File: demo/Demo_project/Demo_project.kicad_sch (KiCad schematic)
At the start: 58 parts, among them J1 USB_C_Receptacle_USB2.0, J2 Conn_01x04, J3 Screw_Terminal_01x03, J4 Screw_Terminal_01x08, J5 Screw_Terminal_01x02, K1 RT314A05, Q1 UMH3N, Q2 BC817, SW1 SW_SPST, U1 ESP32-WROOM-32D, U2 USBLC6-2P6, U3 CP2104, U4 Si7021-A20, U5 74AHCT245, U6 TLV1117LV-3.3

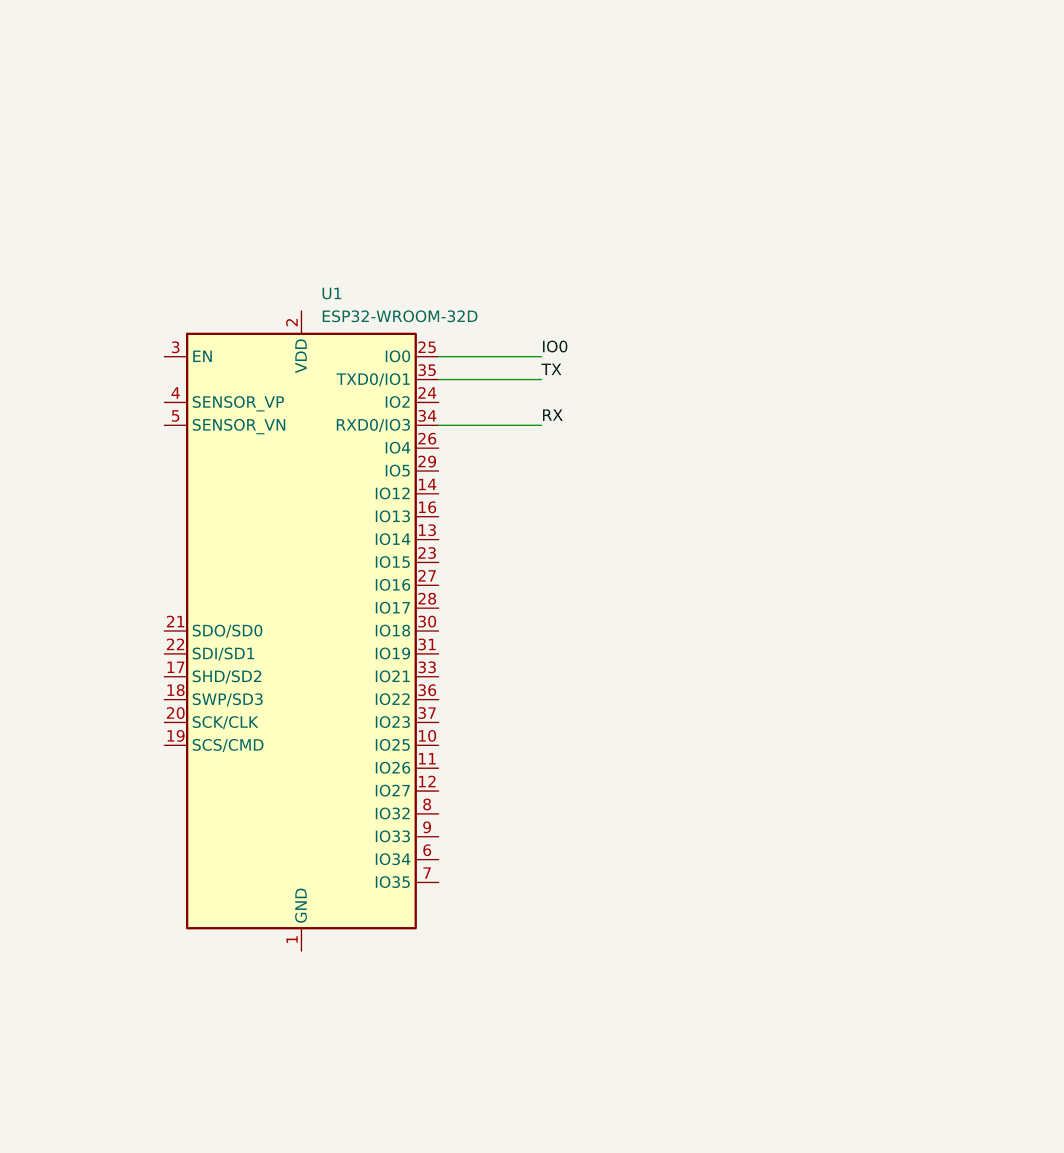
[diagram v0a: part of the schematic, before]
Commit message: v0.1 beta
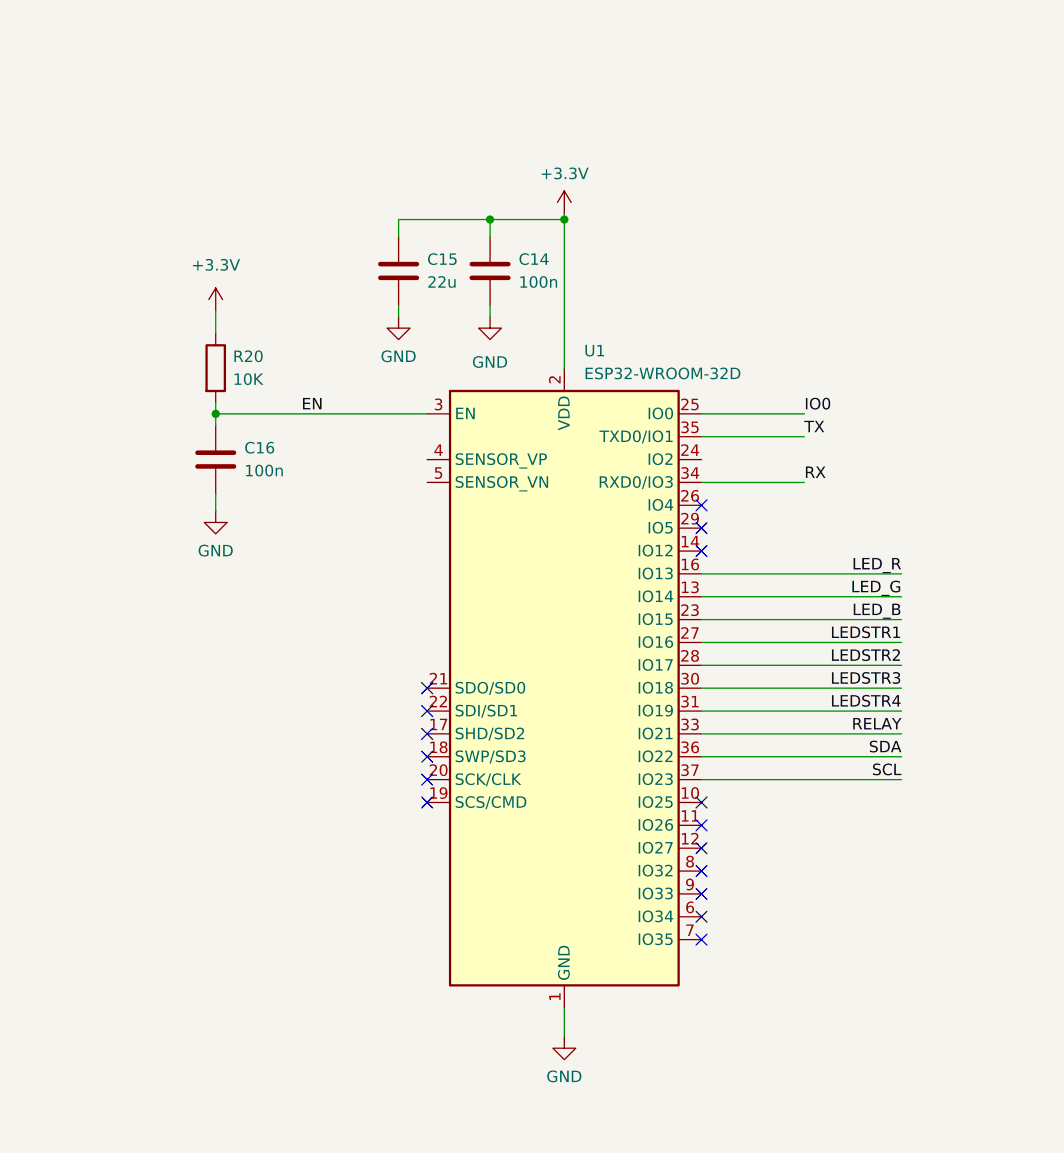
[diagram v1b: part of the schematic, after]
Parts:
- added C14, C16: 100n, symbol Device:C
- added C15: 22u, symbol Device:C
- added R20: 10K, symbol Device:R
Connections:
- net +3.3V: now also U1.2 (VDD), C14.1, C15.1, R20.1
- net EN: now also U1.3 (EN), C16.1, R20.2
- net GND: now also U1.1 (GND), U1.15 (GND), U1.38 (GND), U1.39 (GND), C14.2, C15.2, C16.2
- net LEDSTR1: now also U1.27 (IO16)
- net LEDSTR2: now also U1.28 (IO17)
- net LEDSTR3: now also U1.30 (IO18)
- net LEDSTR4: now also U1.31 (IO19)
- net LED_B: now also U1.23 (IO15)
- net LED_G: now also U1.13 (IO14)
- net LED_R: now also U1.16 (IO13)
- net RELAY: now also U1.33 (IO21)
- net SCL: now also U1.37 (IO23)
- net SDA: now also U1.36 (IO22)
- no-connect marks 4 -> 20
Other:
- moved on the sheet: U1
